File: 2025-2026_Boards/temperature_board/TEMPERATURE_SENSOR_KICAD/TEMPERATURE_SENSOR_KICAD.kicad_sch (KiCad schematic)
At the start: 59 parts, among them J1 LCD Connector Pinout, U1 STM32G431CBT6, U2 TMP235A4DBZR, U3 AMS1117-3.3, U5 TPS62932DRLR, U8 AMS1117

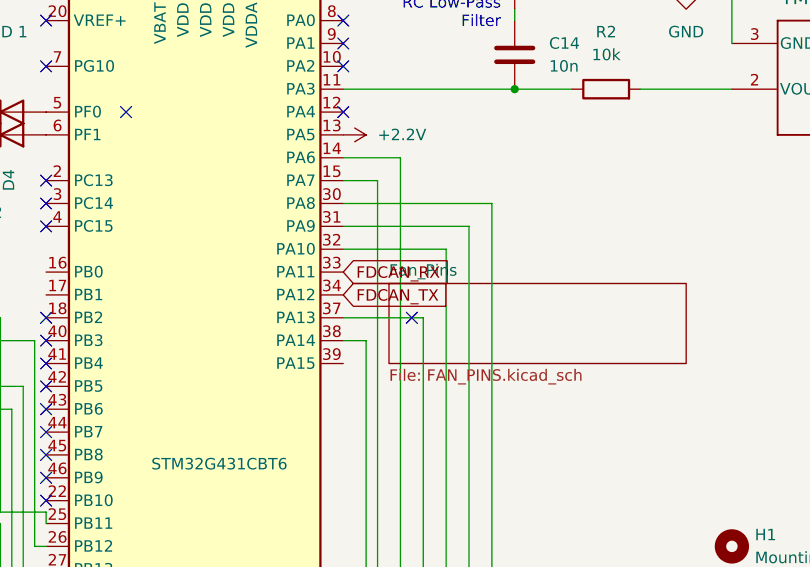
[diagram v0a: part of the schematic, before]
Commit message: updates
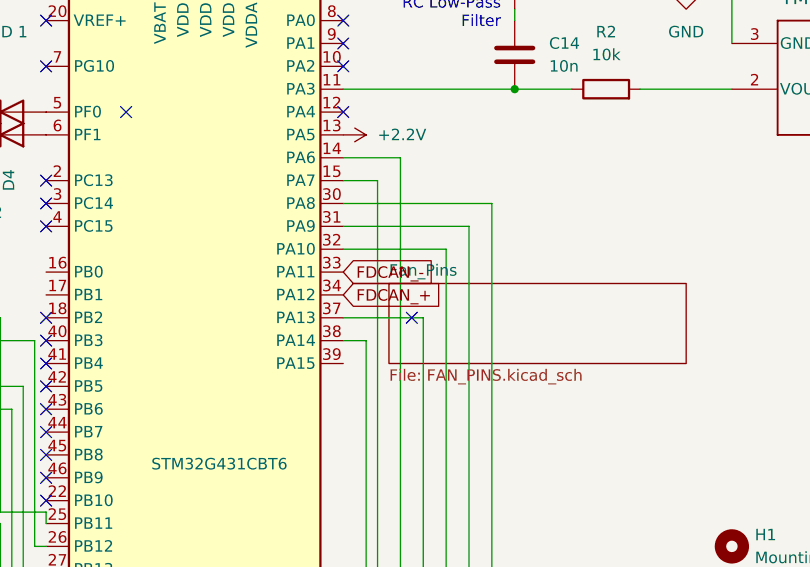
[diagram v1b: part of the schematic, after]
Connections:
- net FDCAN_RX renamed FDCAN_-
- net FDCAN_TX renamed FDCAN_+
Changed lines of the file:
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@@
 		)
 	)
-	(global_label "FDCAN_TX"
+	(global_label "FDCAN_+"
 		(shape input)
 		(at 93.98 113.03 0)
@@
 		)
 		(property "Intersheetrefs" "${INTERSHEET_REFS}"
-			(at 106.1576 113.03 0)
+			(at 105.5529 113.03 0)
 			(effects
 				(font
@@
 		)
 	)
-	(global_label "FDCAN_RX"
+	(global_label "FDCAN_-"
 		(shape input)
 		(at 93.98 110.49 0)
@@
 		)
 		(property "Intersheetrefs" "${INTERSHEET_REFS}"
-			(at 106.46 110.49 0)
+			(at 105.5529 110.49 0)
 			(effects
 				(font
